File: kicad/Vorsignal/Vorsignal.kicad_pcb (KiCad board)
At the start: 2 copper layers, 6.6 x 10.8 mm, 7 parts, among them J0 VCC, J1 VkzBw, J3 GELB, J4 GRÜN

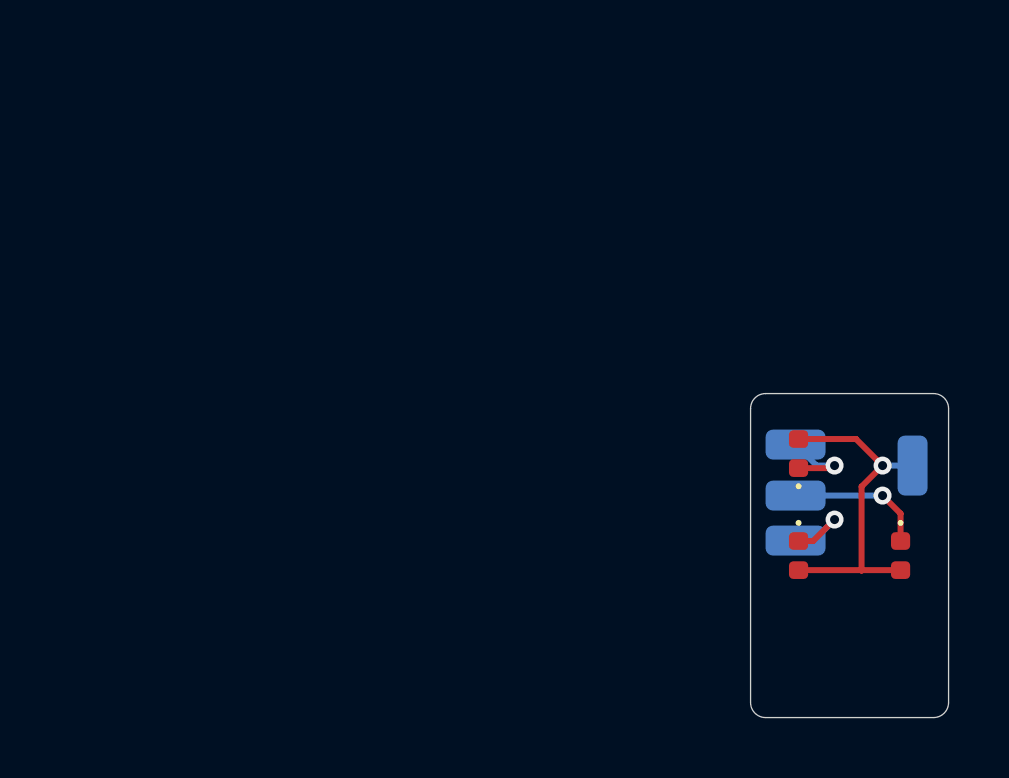
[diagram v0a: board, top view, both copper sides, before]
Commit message: Add CC-BY-SA 4.0 license
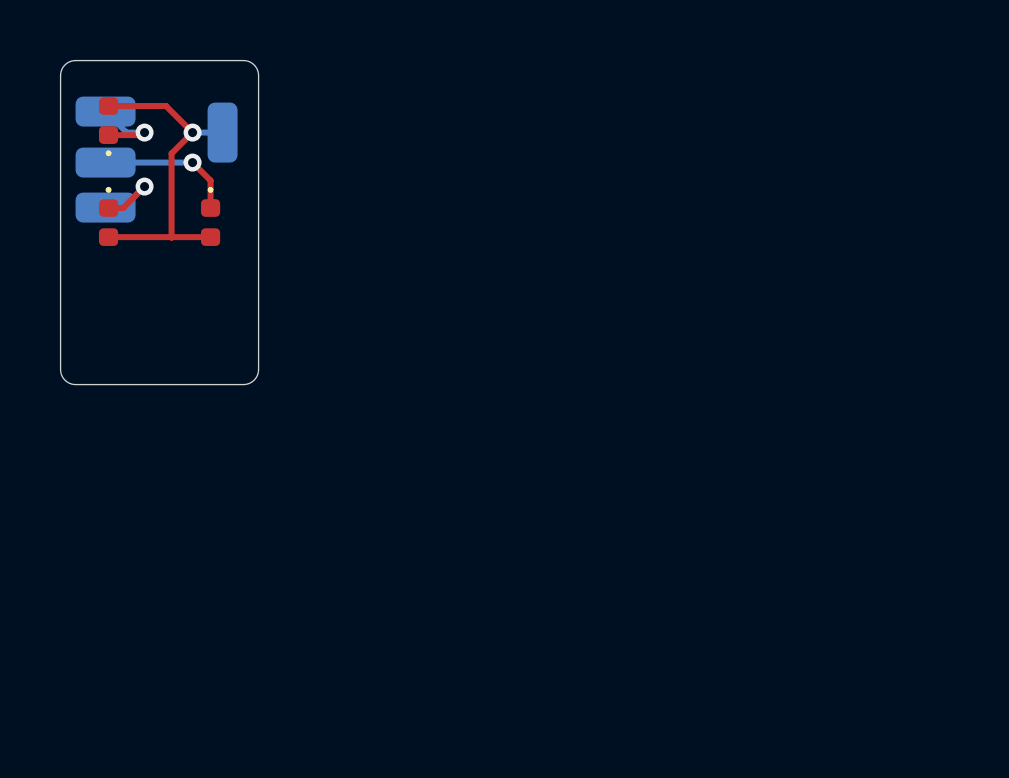
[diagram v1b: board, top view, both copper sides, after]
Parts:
- moved D3 25.5 mm to (98.6, 70.1)
- moved D5 25.5 mm to (102.0, 70.1)
- moved J0 25.5 mm to (102.4, 67.1)
- moved J3 25.5 mm to (98.5, 68.1)
- moved J4 25.5 mm to (98.5, 69.6)
- moved D1 25.5 mm to (98.6, 66.7)
- moved J1 25.5 mm to (98.5, 66.4)
